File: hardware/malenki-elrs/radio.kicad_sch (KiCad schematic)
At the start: 14 parts, among them U3 SX1280IMLTRT, Y2 CRYSTAL 52MHz 10pF SMD

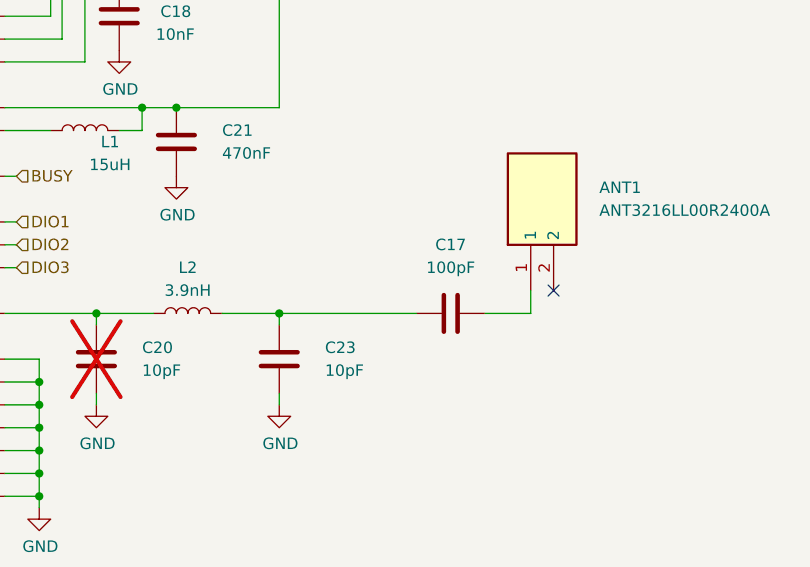
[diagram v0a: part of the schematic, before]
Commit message: minor changes ready for final checks
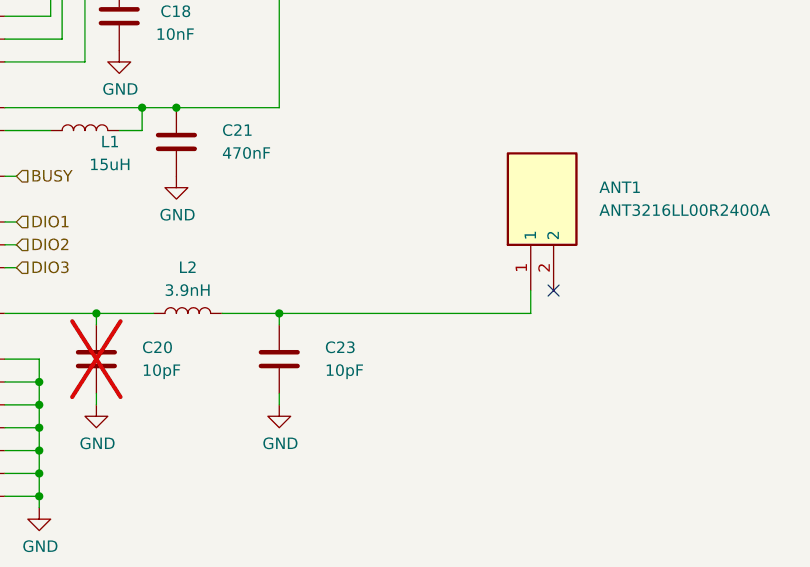
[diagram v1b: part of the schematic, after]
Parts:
- removed C17: 100pF, Capacitor_SMD:C_0402_1005Metric, symbol Device:C
- C16, C19, C22: LCSC (none) -> C100072
- C18: LCSC (none) -> C15195
- C20, C23: LCSC (none) -> C161520
- C21: LCSC (none) -> C92361
- L1: LCSC (none) -> C383402
- L2: LCSC (none) -> C1330553
- R15: LCSC C25744 -> C71617; Manufacturer Uniroyal -> VISHAY; Partnum C25804 -> CRCW040210K0FKED
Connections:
- net at C23.1, L2.2: now also ANT1.1
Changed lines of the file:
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@@
-	(wire
-		(pts
-			(xy 196.85 121.92) (xy 201.93 121.92)
-		)
-		(stroke
-			(width 0)
-			(type default)
-		)
-	)
 	(wire
 		(pts
@@
 	(wire
 		(pts
-			(xy 173.99 121.92) (xy 189.23 121.92)
+			(xy 173.99 121.92) (xy 201.93 121.92)
 		)
 		(stroke
@@
 			)
 		)
+		(property "LCSC" "C100072"
+			(at 171.45 67.31 0)
+			(hide yes)
+			(show_name no)
+			(do_not_autoplace no)
+			(effects
+				(font
+					(size 1.27 1.27)
+				)
+			)
+		)
 		(pin "2"
 		)
@@
 			)
 		)
+		(property "LCSC" "C1330553"
+			(at 163.83 121.92 90)
+			(hide yes)
+			(show_name no)
+			(do_not_autoplace no)
+			(effects
+				(font
+					(size 1.27 1.27)
+				)
+			)
+		)
 		(pin "2"
 		)
@@
 		)
 		(property "Description" "Unpolarized capacitor"
+			(at 138.43 67.31 0)
+			(hide yes)
+			(show_name no)
+			(do_not_autoplace no)
+			(effects
+				(font
+					(size 1.27 1.27)
+				)
+			)
+		)
+		(property "LCSC" "C100072"
 			(at 138.43 67.31 0)
 			(hide yes)
@@
 			)
 		)
+		(property "LCSC" "C161520"
+			(at 173.99 127 0)
+			(hide yes)
+			(show_name no)
+			(do_not_autoplace no)
+			(effects
+				(font
+					(size 1.27 1.27)
+				)
+			)
+		)
 		(pin "2"
 		)
@@
 			)
 		)
+		(property "LCSC" "C15195"
+			(at 156.21 88.9 0)
+			(hide yes)
+			(show_name no)
+			(do_not_autoplace no)
+			(effects
+				(font
+					(size 1.27 1.27)
+				)
+			)
+		)
 		(pin "2"
 		)
@@
 			)
 		)
-		(property "Datasheet" ""
+		(property "Datasheet" "https://www.lcsc.com/datasheet/C71617.pdf?spm=wm.sxq.inf.ggs___wm.fly.bg.2.xh&lcsc_vid=FVleV1NXFQNYX1VeQQVdBFdRRgJeVQZfEgAMBQBUQVAxVlNRQFBZU1RfQ1VdVzsOAxUeFF5JWBYZEEoKFBINSQcJGk4eFQsCAgIaSgADAwAHC0slTlFbUkoOAwwC"
 			(at 101.6 92.71 0)
 			(hide yes)
@@
 			)
 		)
-		(property "Description" ""
+		(property "Description" "63mW 10kΩ 50V Thick Film Resistor ±1% ±100ppm/℃ 0402 Chip Resistor - Surface Mount RoHS"
 			(at 101.6 92.71 0)
 			(hide yes)
@@
 			)
 		)
-		(property "Partnum" "C25804"
+		(property "Partnum" "CRCW040210K0FKED"
 			(at 101.6 92.71 0)
 			(hide yes)
@@
 			)
 		)
-		(property "LCSC" "C25744"
+		(property "LCSC" "C71617"
 			(at 101.6 92.71 0)
 			(hide yes)
@@
 			)
 		)
-		(property "Manufacturer" "Uniroyal"
+		(property "Manufacturer" "VISHAY"
 			(at 101.6 92.71 0)
 			(hide yes)
@@
 			)
 		)
+		(property "LCSC" "C161520"
+			(at 153.67 127 0)
+			(hide yes)
+			(show_name no)
+			(do_not_autoplace no)
+			(effects
+				(font
+					(size 1.27 1.27)
+				)
+			)
+		)
 		(pin "2"
 		)
@@
 			)
 		)
+		(property "LCSC" "C383402"
+			(at 152.4 101.6 90)
+			(hide yes)
+			(show_name no)
+			(do_not_autoplace no)
+			(effects
+				(font
+					(size 1.27 1.27)
+				)
+			)
+		)
 		(pin "2"
 		)
@@
 	(symbol
 		(lib_id "Device:C")
-		(at 193.04 121.92 90)
-		(unit 1)
-		(body_style 1)
-		(exclude_from_sim no)
-		(in_bom yes)
-		(on_board yes)
-		(in_pos_files yes)
-		(dnp no)
-		(fields_autoplaced yes)
-		(property "Reference" "C17"
-			(at 193.04 114.3 90)
-			(show_name no)
-			(do_not_autoplace no)
-			(effects
-				(font
-					(size 1.27 1.27)
-				)
-			)
-		)
-		(property "Value" "100pF"
-			(at 193.04 116.84 90)
-			(show_name no)
-			(do_not_autoplace no)
-			(effects
-				(font
-					(size 1.27 1.27)
-				)
-			)
-		)
-		(property "Footprint" "Capacitor_SMD:C_0402_1005Metric"
-			(at 196.85 120.9548 0)
-			(hide yes)
-			(show_name no)
-			(do_not_autoplace no)
-			(effects
-				(font
-					(size 1.27 1.27)
-				)
-			)
-		)
-		(property "Datasheet" ""
-			(at 193.04 121.92 0)
-			(hide yes)
-			(show_name no)
-			(do_not_autoplace no)
-			(effects
-				(font
-					(size 1.27 1.27)
-				)
-			)
-		)
-		(property "Description" "Unpolarized capacitor"
-			(at 193.04 121.92 0)
-			(hide yes)
-			(show_name no)
-			(do_not_autoplace no)
-			(effects
-				(font
-					(size 1.27 1.27)
-				)
-			)
-		)
-		(pin "2"
-		)
-		(pin "1"
-		)
-		(instances
-			(project "malenki-elrs"
-				(path "/f41619e3-8cf2-4511-8a51-762d4de43197/f8865f8d-c9c7-4324-8715-db444b940a42"
-					(reference "C17")
-					(unit 1)
-				)
-			)
-		)
-	)
-	(symbol
-		(lib_id "Device:C")
 		(at 154.94 67.31 0)
 		(unit 1)
@@
 		)
 		(property "Description" "Unpolarized capacitor"
+			(at 154.94 67.31 0)
+			(hide yes)
+			(show_name no)
+			(do_not_autoplace no)
+			(effects
+				(font
+					(size 1.27 1.27)
+				)
+			)
+		)
+		(property "LCSC" "C100072"
 			(at 154.94 67.31 0)
 			(hide yes)
@@
 			(at 162.56 102.87 0)
 			(hide yes)
+			(show_name no)
+			(do_not_autoplace no)
+			(effects
+				(font
+					(size 1.27 1.27)
+				)
+			)
+		)
+		(property "LCSC" "C92361"
+			(at 162.56 102.87 0)
+			(hide yes)
